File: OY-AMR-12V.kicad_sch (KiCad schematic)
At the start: 16 parts

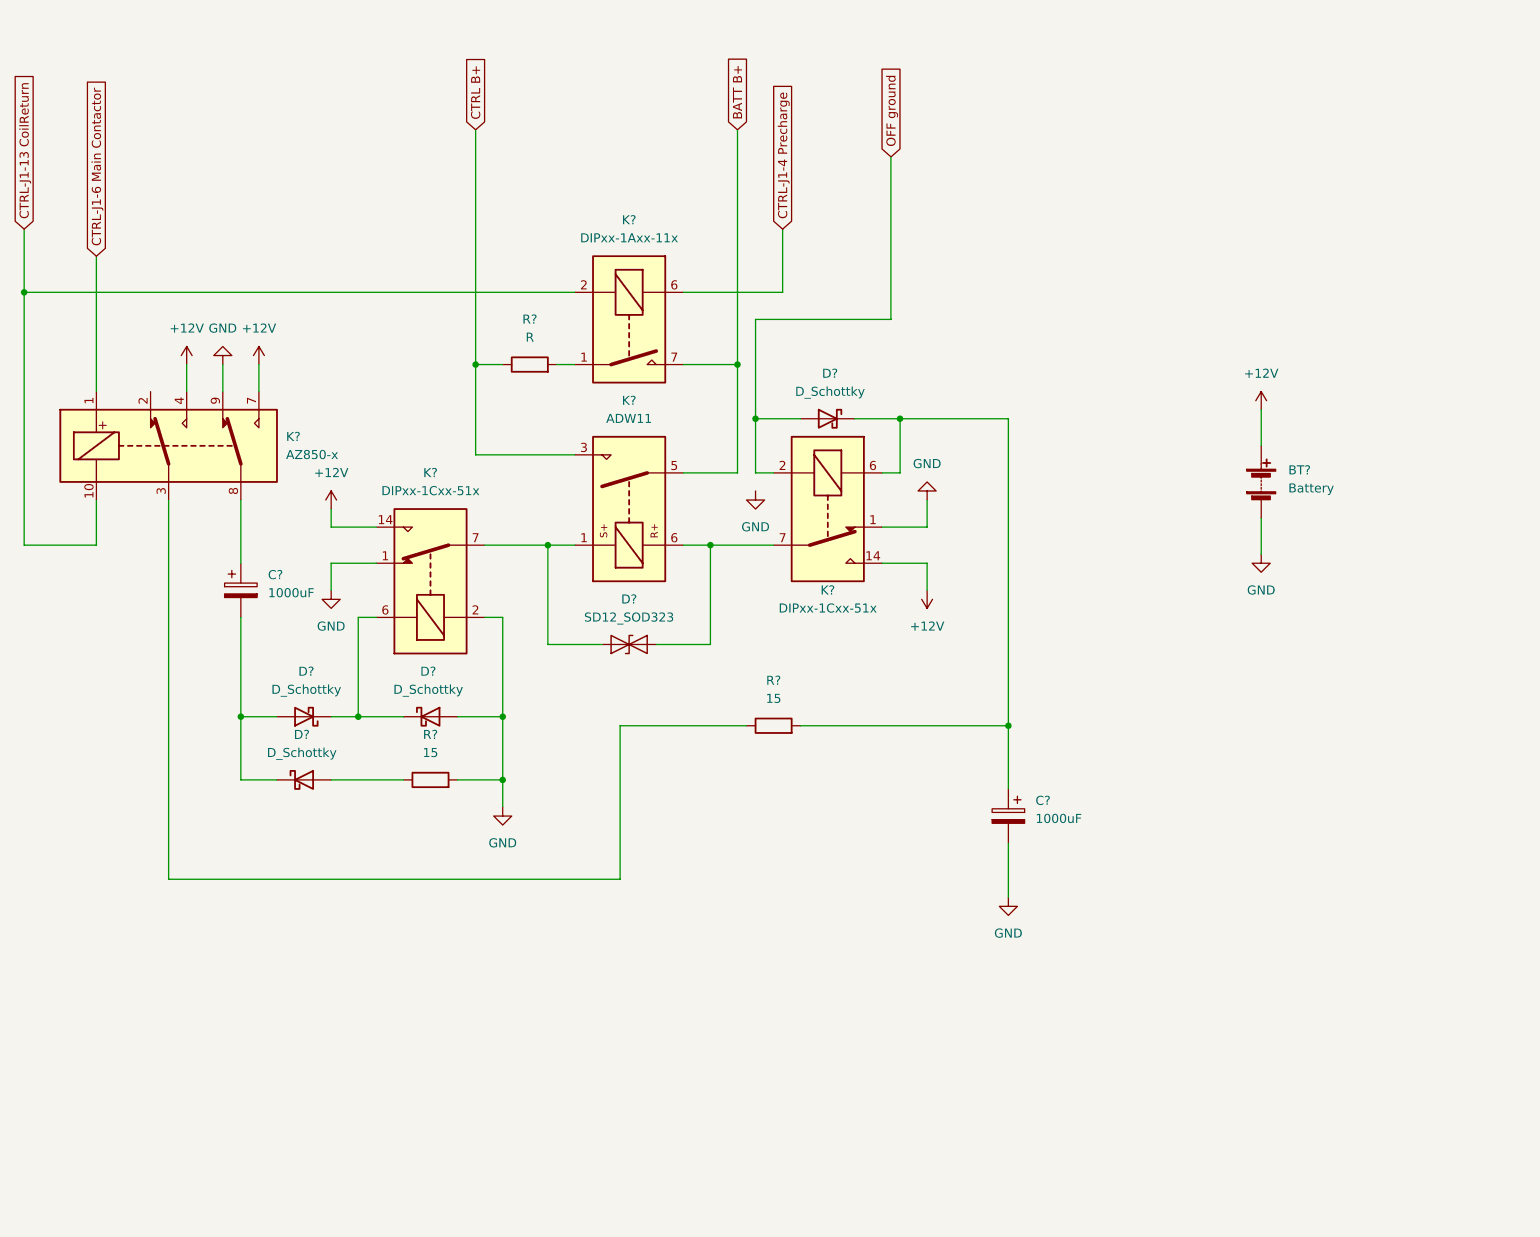
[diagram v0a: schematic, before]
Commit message: Relay-only version in progress
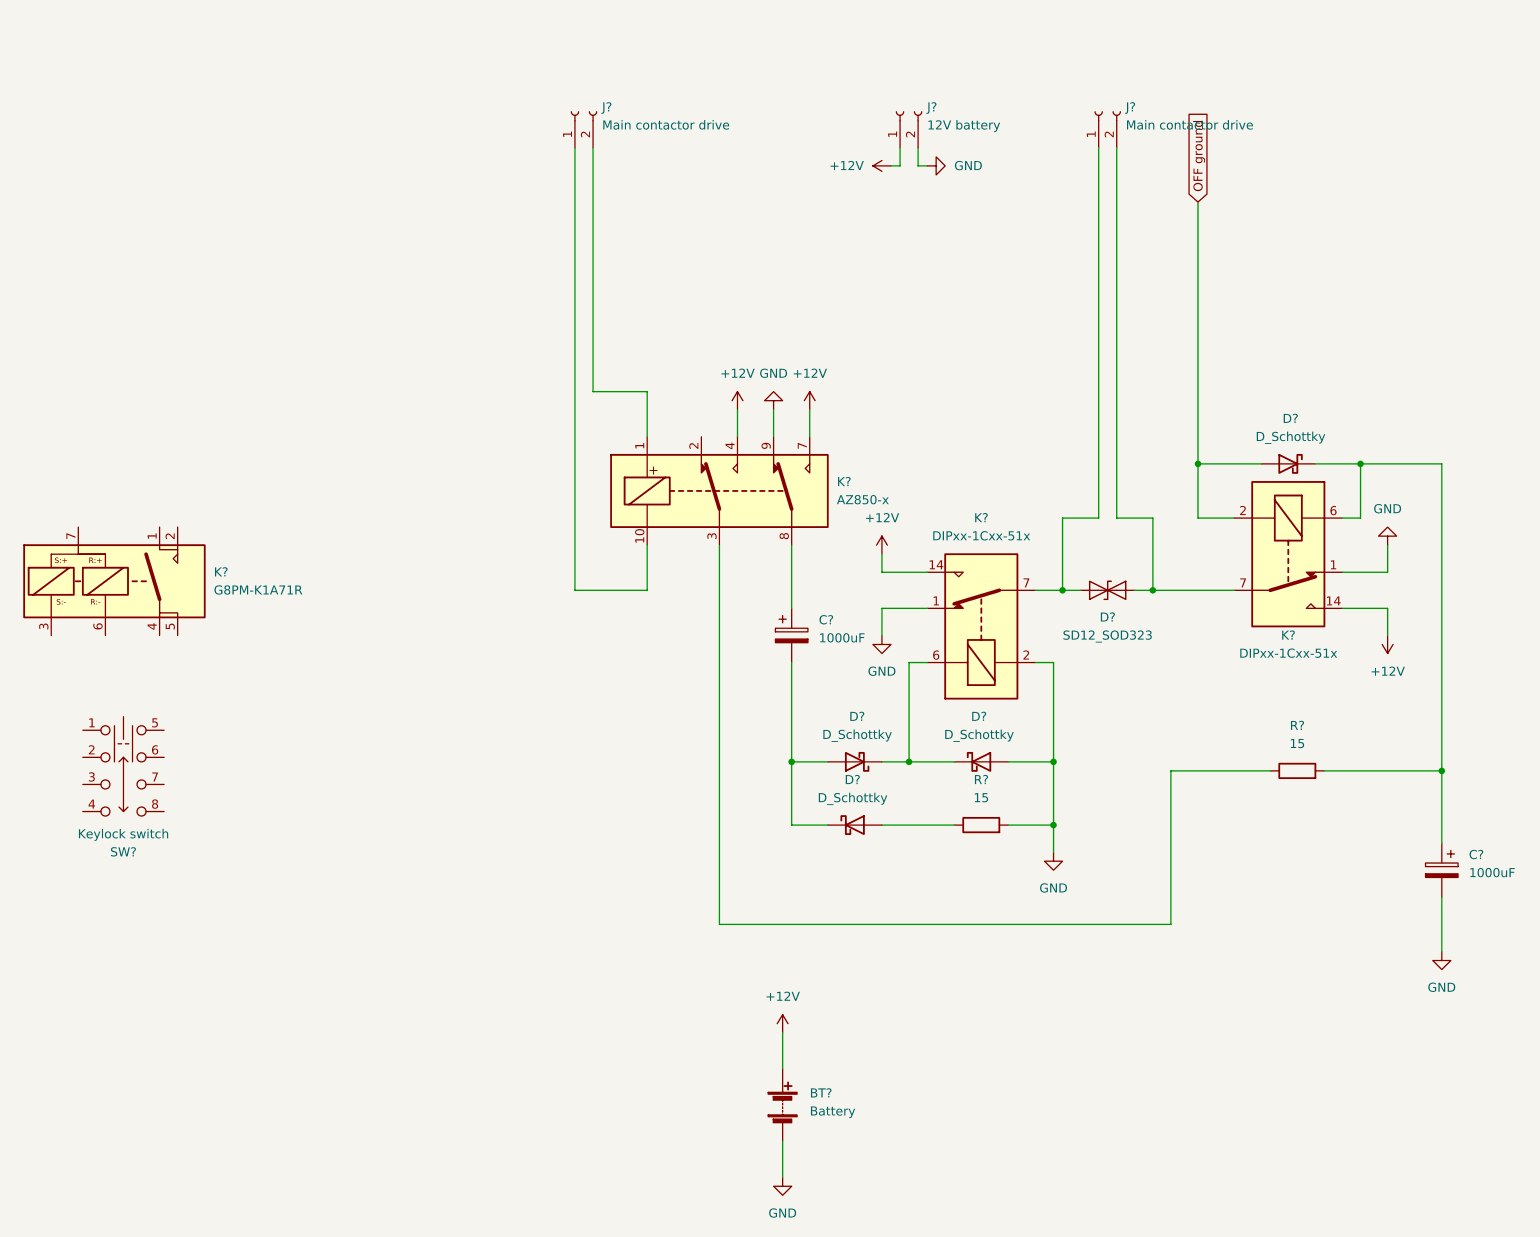
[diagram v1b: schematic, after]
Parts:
- removed K?: ADW11, Relay_THT:Relay_1P1T_NO_10x24x18.8mm_Panasonic_ADW11xxxxW_THT, symbol Relay:ADW11
- removed K?: DIPxx-1Axx-11x, Relay_THT:Relay_StandexMeder_DIP_LowProfile, symbol Relay:DIPxx-1Axx-11x
- removed R?: R, symbol Device:R
- added J? (x2): Main contactor drive, symbol Connector:Conn_01x02_Female
- added J?: 12V battery, symbol Connector:Conn_01x02_Female
- added K?: G8PM-K1A71R, symbol Miscellaneous:G8PM-K1A71R
- added SW?: Keylock switch, symbol Miscellaneous:H200AA2F205NQ
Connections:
- net +12V: now also J?.1 (Pin_1)
- net GND: now also J?.2 (Pin_2)
- net at D?.1 (A1), K?.7, K?.8: now also J?.1 (Pin_1)
- net at D?.2 (A2), K?.7, K?.8: now also J?.2 (Pin_2)
- net CTRL-J1-13 CoilReturn: no longer names the net of K?.10
- net CTRL-J1-13 CoilReturn: now also J?.1 (Pin_1)
- net CTRL-J1-6 Main Contactor: no longer names the net of K?.1
- net CTRL-J1-6 Main Contactor: now also J?.2 (Pin_2)
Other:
- moved on the sheet: BT?, C?, D?, K?, R?
